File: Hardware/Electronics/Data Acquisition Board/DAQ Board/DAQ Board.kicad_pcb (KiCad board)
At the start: 4 copper layers, 94.7 x 58.9 mm, 170 parts, among them J1 Conn_01x09_Male, J10 ~CS~_TP, J12 START_TP, J14 MID_SUPPLY_TP, J15 AVDD_TP, J16 DVDD_TP, J2 USB_B_Mini, J3 Battery Connector, J4 DC Barrel Jack, J5 HC-05 BT Module, J6 ICSP Header, J7 VIN_RAW_TP, Q1 DMP2100U, SW1 DIP, SW10 SW_SPDT, SW11 SW_SPDT, SW2 SW_DIP_x02, SW3 SW_SPDT, SW4 SW_SPDT, SW5 SW_SPDT, SW6 SW_SPDT, SW7 SW_SPDT, SW8 SW_SPDT, SW9 SW_SPDT, U1 ATmega328P-AU, U2 MCP1755T-5002E_SOT223-5, U3 LM3480-3.3, U4 MCP1755T-5002E_SOT223-5, U5 FT232RL, Y1 16MHz

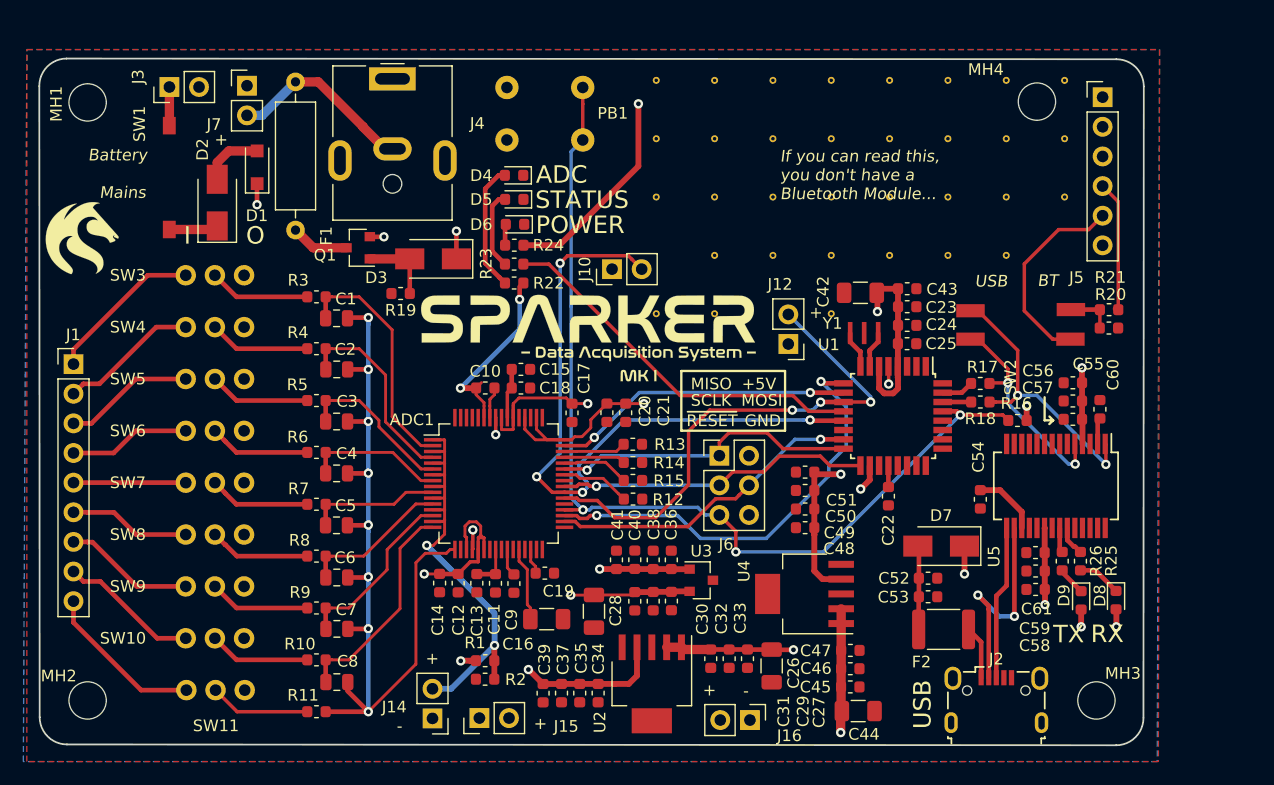
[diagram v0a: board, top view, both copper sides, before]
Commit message: Many changes, mostly about rotating the board
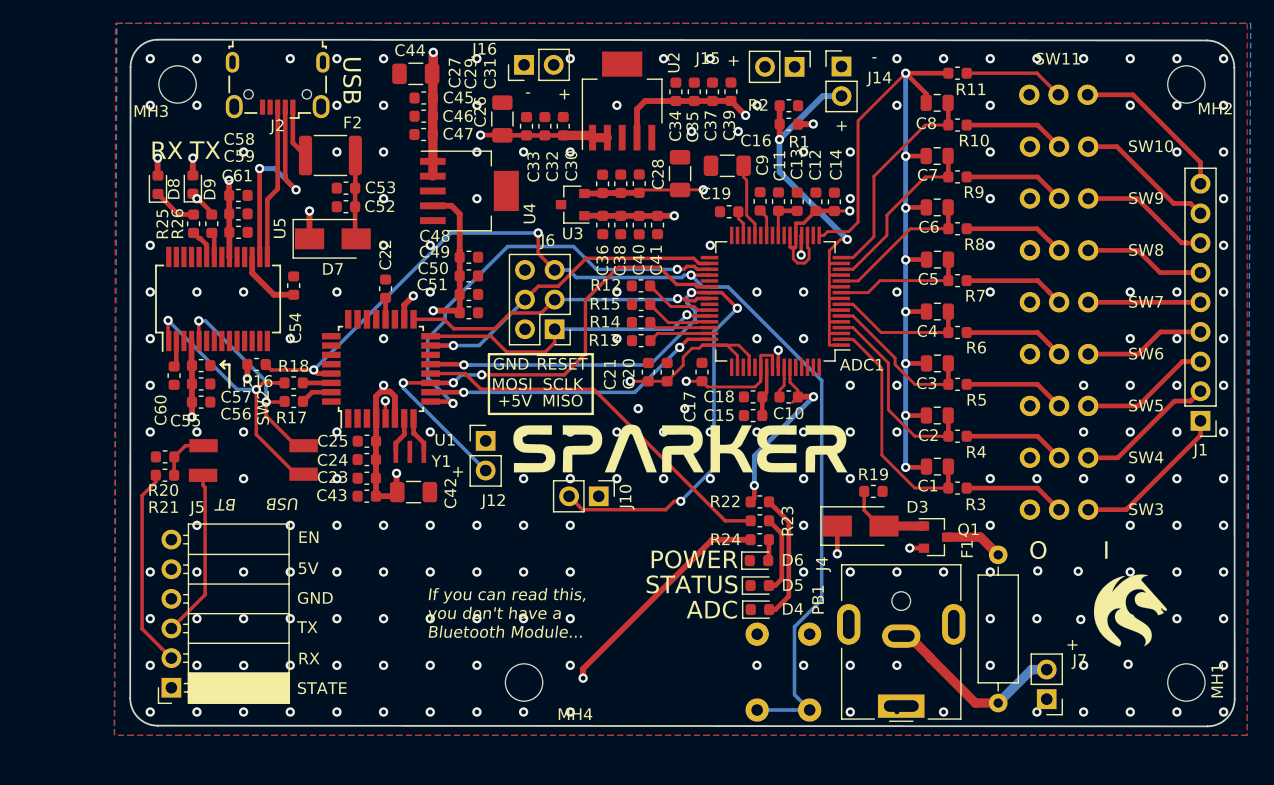
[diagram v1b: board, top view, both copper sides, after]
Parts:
- removed ? (x33): , Vias:VIA-0.6mm
- removed D1: NSR20F40NXT5GOSCT-ND, Diode_SMD:D_SOD-123F
- removed D2: MURA140T3GOSCT-ND, Diode_SMD:D_SMA
- removed J3: Battery Connector, Connector_PinHeader_2.54mm:PinHeader_1x02_P2.54mm_Vertical
- removed SW1: DIP, Switches:DIP-Switch_01x01
- removed TEXT1: Text, Sparker:NASA_subtext
- moved MH2 108.0 mm to (216.8, 70.8), turned to 180 degrees
- moved MH1 106.5 mm to (216.8, 122.1), turned to 180 degrees
- moved J1 96.7 mm to (218.0, 99.7), turned to 180 degrees
- moved LOGO1 95.4 mm to (212.0, 116.0)
- moved MH3 94.8 mm to (130.4, 70.8), turned to 180 degrees
- moved J5 94.5 mm to (129.8, 122.5), turned to 180 degrees
- moved D8 89.5 mm to (128.7, 79.4), turned to 90 degrees
- moved J7 86.4 mm to (204.9, 123.5), turned to 180 degrees
- moved SW11 84.4 mm to (203.4, 71.7), turned to 0 degrees
- moved D9 84.1 mm to (131.7, 79.4), turned to 90 degrees
- moved R21 82.2 mm to (129.3, 104.3), turned to 0 degrees
- moved R20 81.6 mm to (129.3, 102.8), turned to 180 degrees
- moved R25 81.3 mm to (131.7, 82.8), turned to 270 degrees
- moved J2 81.1 mm to (138.9, 70.9), turned to 180 degrees
- moved SW10 79.5 mm to (203.4, 76.2), turned to 0 degrees
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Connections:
- J5 pad 2: /+5V -> /HC05_TX
- J5 pad 3: /GND -> /HC05_RX
- J5 pad 4: /HC05_RX -> /GND
- J5 pad 5: /HC05_TX -> /+5V
- R21 pad 1: /HC05_RX -> /HC05_TX
- SW2 pad 3: /HC05_TX -> Net-(R20-Pad1)
- SW2 pad 4: Net-(R20-Pad1) -> /HC05_RX
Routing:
- net /~RESET: track 84.5 -> 96.6 mm
- net /VBAT: track 5.27 -> 0.00 mm
- net Net-(D2-Pad1): track 4.23 -> 0.00 mm
- net Net-(J3-Pad1): track 3.31 -> 0.00 mm
- net /HC05_RX: track 11.4 -> 14.4 mm
- net /~CS: track 58.5 -> 60.5 mm
- net /VIN: track 27.3 -> 25.4 mm, vias 5 -> 4
- net /+5V: track 69.6 -> 71.4 mm
- net Net-(R20-Pad1): track 4.05 -> 5.14 mm
- net Net-(D3-Pad2): track 6.39 -> 7.30 mm
- net /HC05_TX: track 18.1 -> 17.4 mm
- net /GND: track 4.68 -> 4.69 mm, vias 3 -> 205
- net Net-(D9-Pad1): vias 0 -> 1
- net (no net): vias 0 -> 1
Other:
- outline, holes or cut-outs redrawn
- board text removed: "Battery"
- board text removed: "Mains"
